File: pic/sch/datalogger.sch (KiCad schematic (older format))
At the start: 18 parts

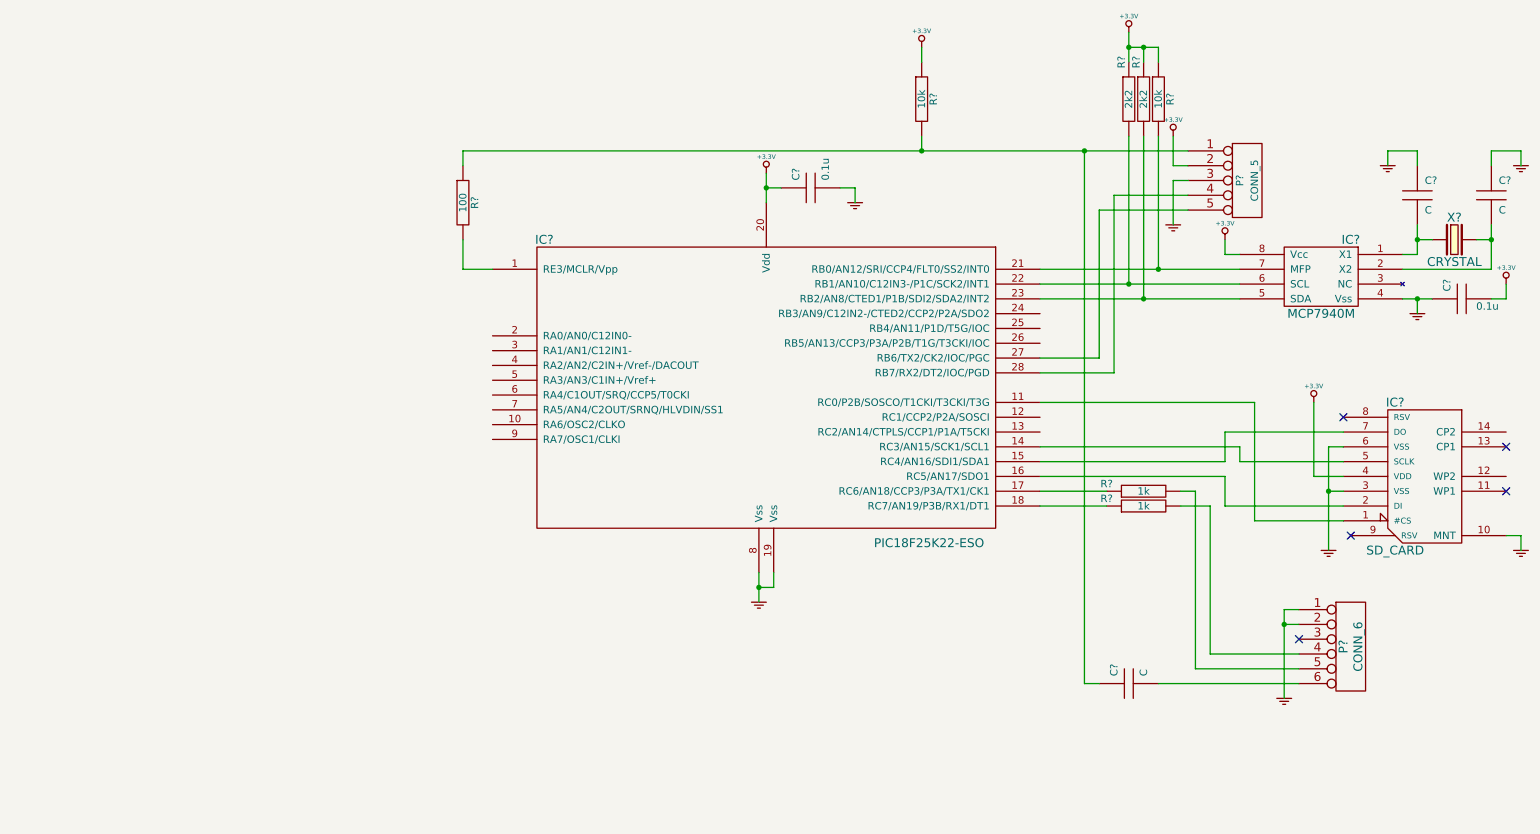
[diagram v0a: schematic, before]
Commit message: More schematic tweaks. Almost ready for PCB
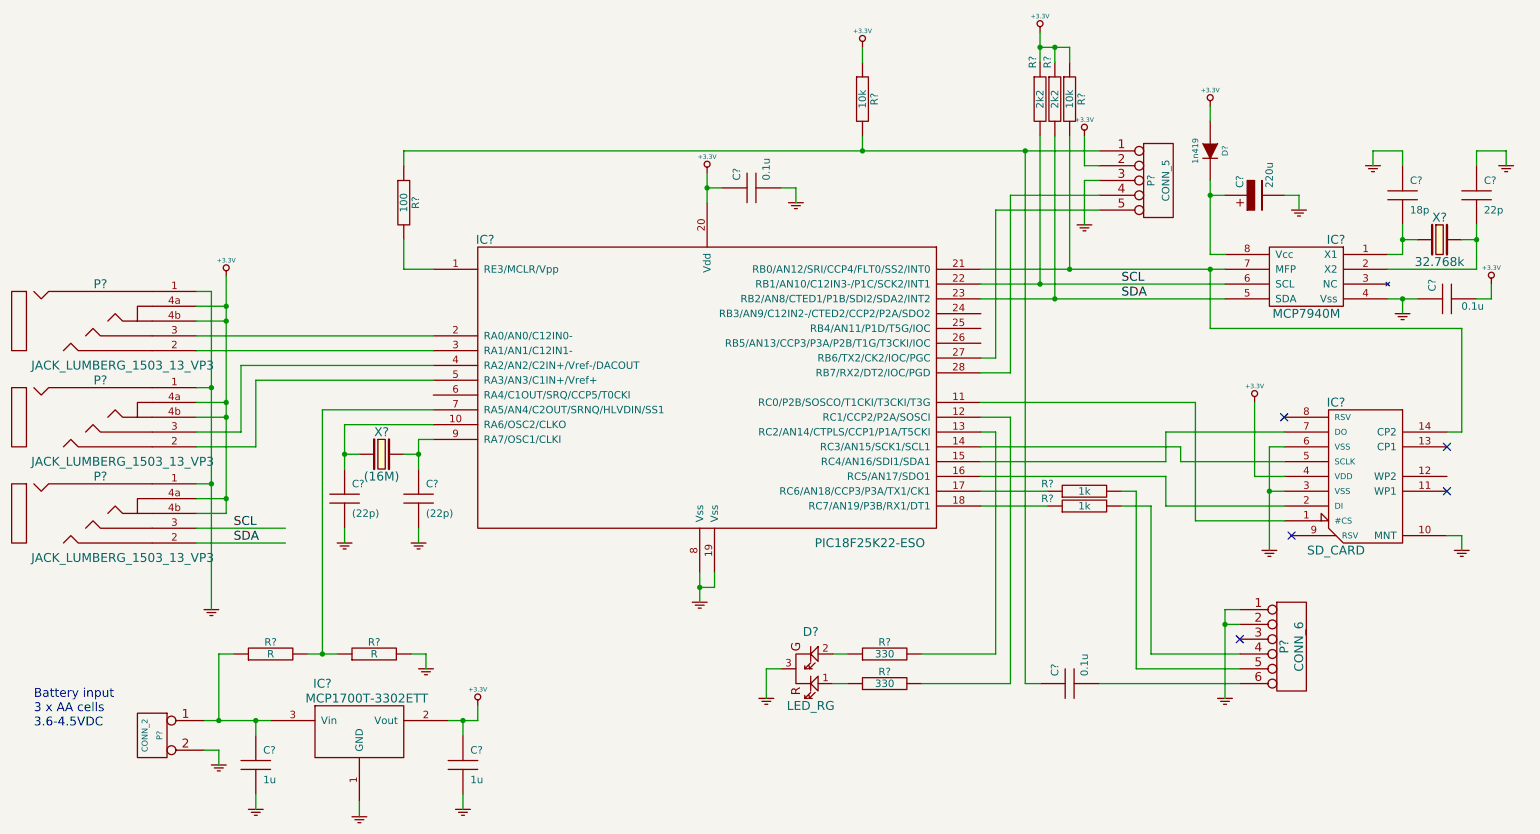
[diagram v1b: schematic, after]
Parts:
- added C? (x2): (22p), symbol C
- added C?: 220u, symbol CAPAPOL
- added C? (x2): 1u, symbol C
- added D?: LED_RG, symbol LED_RG
- added D?: 1n419, symbol DIODE
- added IC?: MCP1700T-3302ETT, symbol MCP1700T-3302ETT
- added P? (x3): JACK_LUMBERG_1503_13_VP3, symbol JACK_LUMBERG_1503_13_VP3
- added P?: CONN_2, symbol CONN_2
- added R? (x2): 330, symbol R
- added R? (x2): R, symbol R
- added X?: (16M), symbol CRYSTAL
- C?: value C -> 18p
- C?: value C -> 22p
- C?: value C -> 0.1u
- X?: value CRYSTAL -> 32.768k
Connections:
- net +3.3V: now also C?.1, D?.1 (A), IC?.2 (Vout), P?.4a, P?.4a, P?.4a, P?.4b, P?.4b, P?.4b; no longer IC?.8 (Vcc)
- net GND: now also C?.2, C?.2, C?.2, C?.2, C?.2, D?.3 (GND), IC?.1 (GND), P?.1, P?.1, P?.1, P?.2 (PM), R?.2
- net at IC?.10 (RA6/OSC2/CLKO): now also C?.1, X?.1
- net at IC?.12 (RC1/CCP2/P2A/SOSCI): now also R?.2
- net at IC?.13 (RC2/AN14/CTPLS/CCP1/P1A/T5CKI): now also R?.2
- net at IC?.2 (RA0/AN0/C12IN0-): now also P?.3
- net at IC?.21 (RB0/AN12/SRI/CCP4/FLT0/SS2/INT0), IC?.7 (MFP), R?.2: now also IC?.14 (CP2)
- net SCL: now reaches IC?.22 (RB1/AN10/C12IN3-/P1C/SCK2/INT1), IC?.6 (SCL), R?.2
- net SCL: now also P?.3
- net SDA: now reaches IC?.23 (RB2/AN8/CTED1/P1B/SDI2/SDA2/INT2), IC?.5 (SDA), R?.2
- net SDA: now also P?.2
- net at IC?.3 (RA1/AN1/C12IN1-): now also P?.2
- net at IC?.4 (RA2/AN2/C2IN+/Vref-/DACOUT): now also P?.3
- net at IC?.5 (RA3/AN3/C1IN+/Vref+): now also P?.2
- net at IC?.7 (RA5/AN4/C2OUT/SRNQ/HLVDIN/SS1): now also R?.1, R?.2
- net at IC?.9 (RA7/OSC1/CLKI): now also C?.1, X?.2
- new net: C?.1, D?.2 (K), IC?.8 (Vcc)
- new net: D?.1 (RED), R?.1
- new net: D?.2 (GRN), R?.1
- new net: C?.1, IC?.3 (Vin), P?.1 (P1), R?.1
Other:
- note added: "Battery input\n3 x AA cells\n3.6-4.5VDC"
- moved on the sheet: C?, IC?, P?, R?, X?
